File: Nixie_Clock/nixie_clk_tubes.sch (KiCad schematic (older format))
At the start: 20 parts, among them Y1 IN-14, Y2 IN-14, Y3 IN-14, Y4 IN-14, Y5 IN-14, Y6 IN-14, Y7 nixie_colon, Y8 nixie_colon

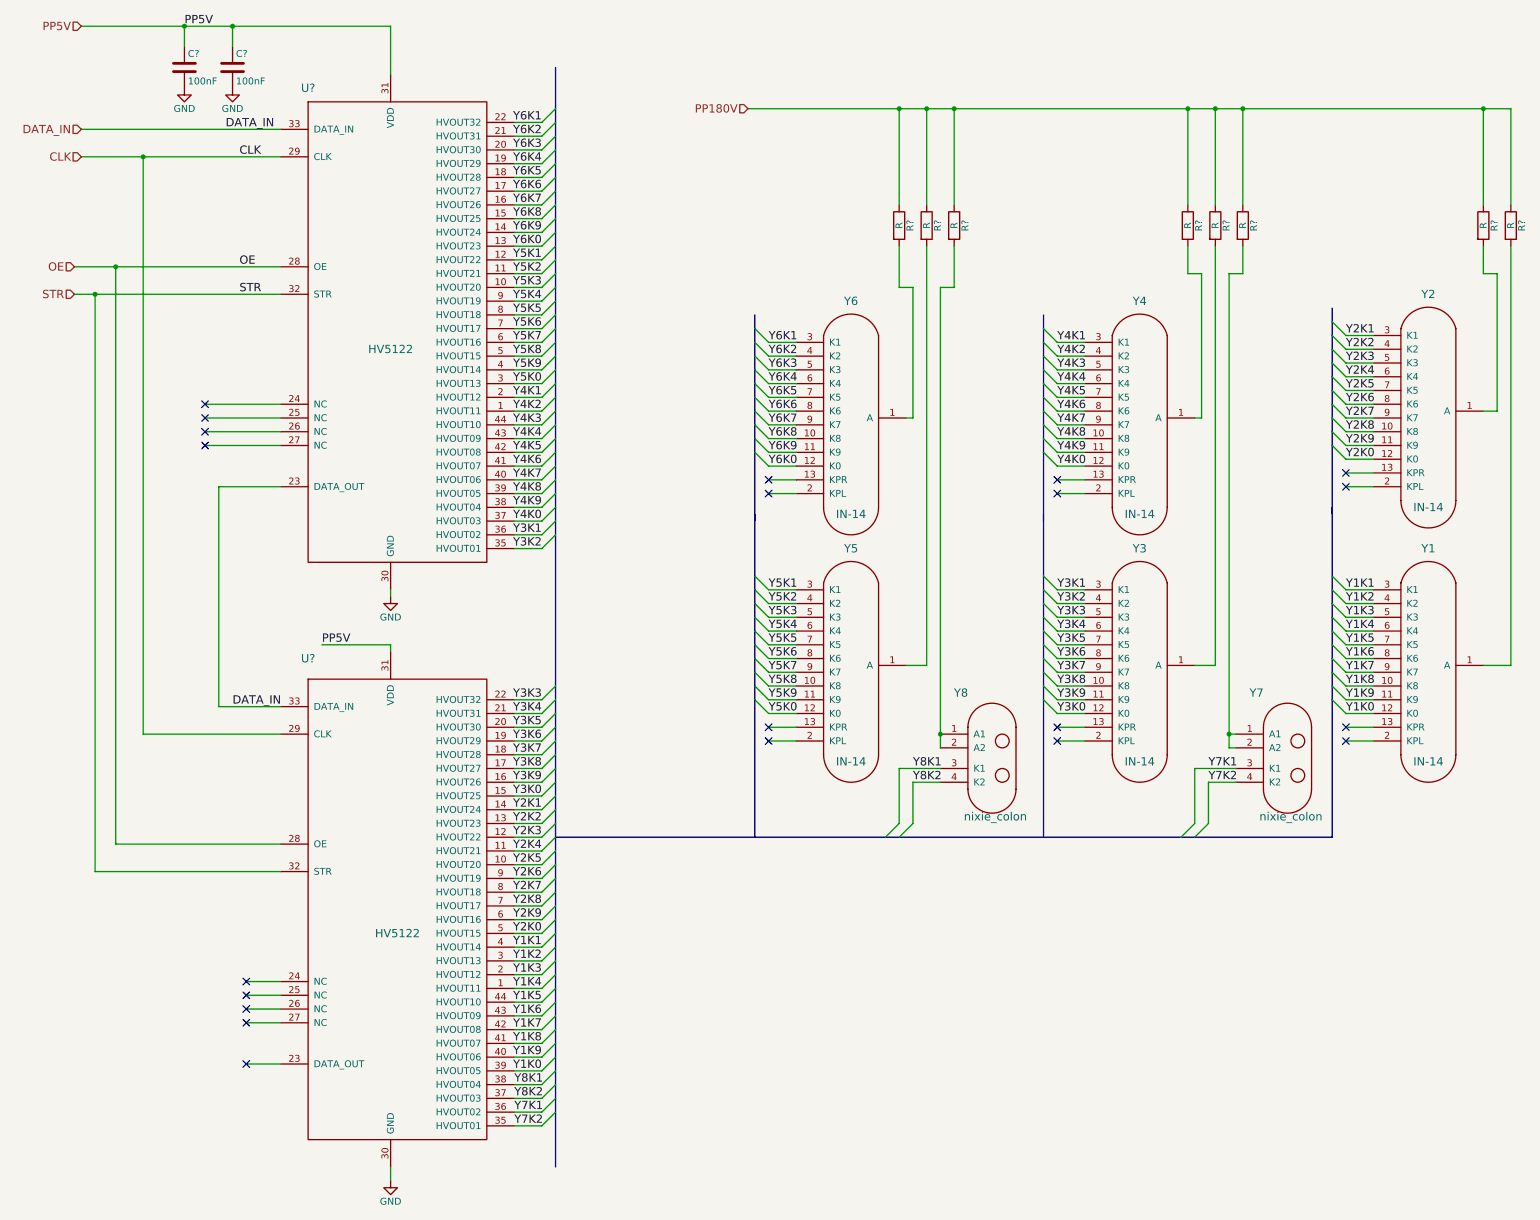
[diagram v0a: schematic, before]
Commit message: Sync remote
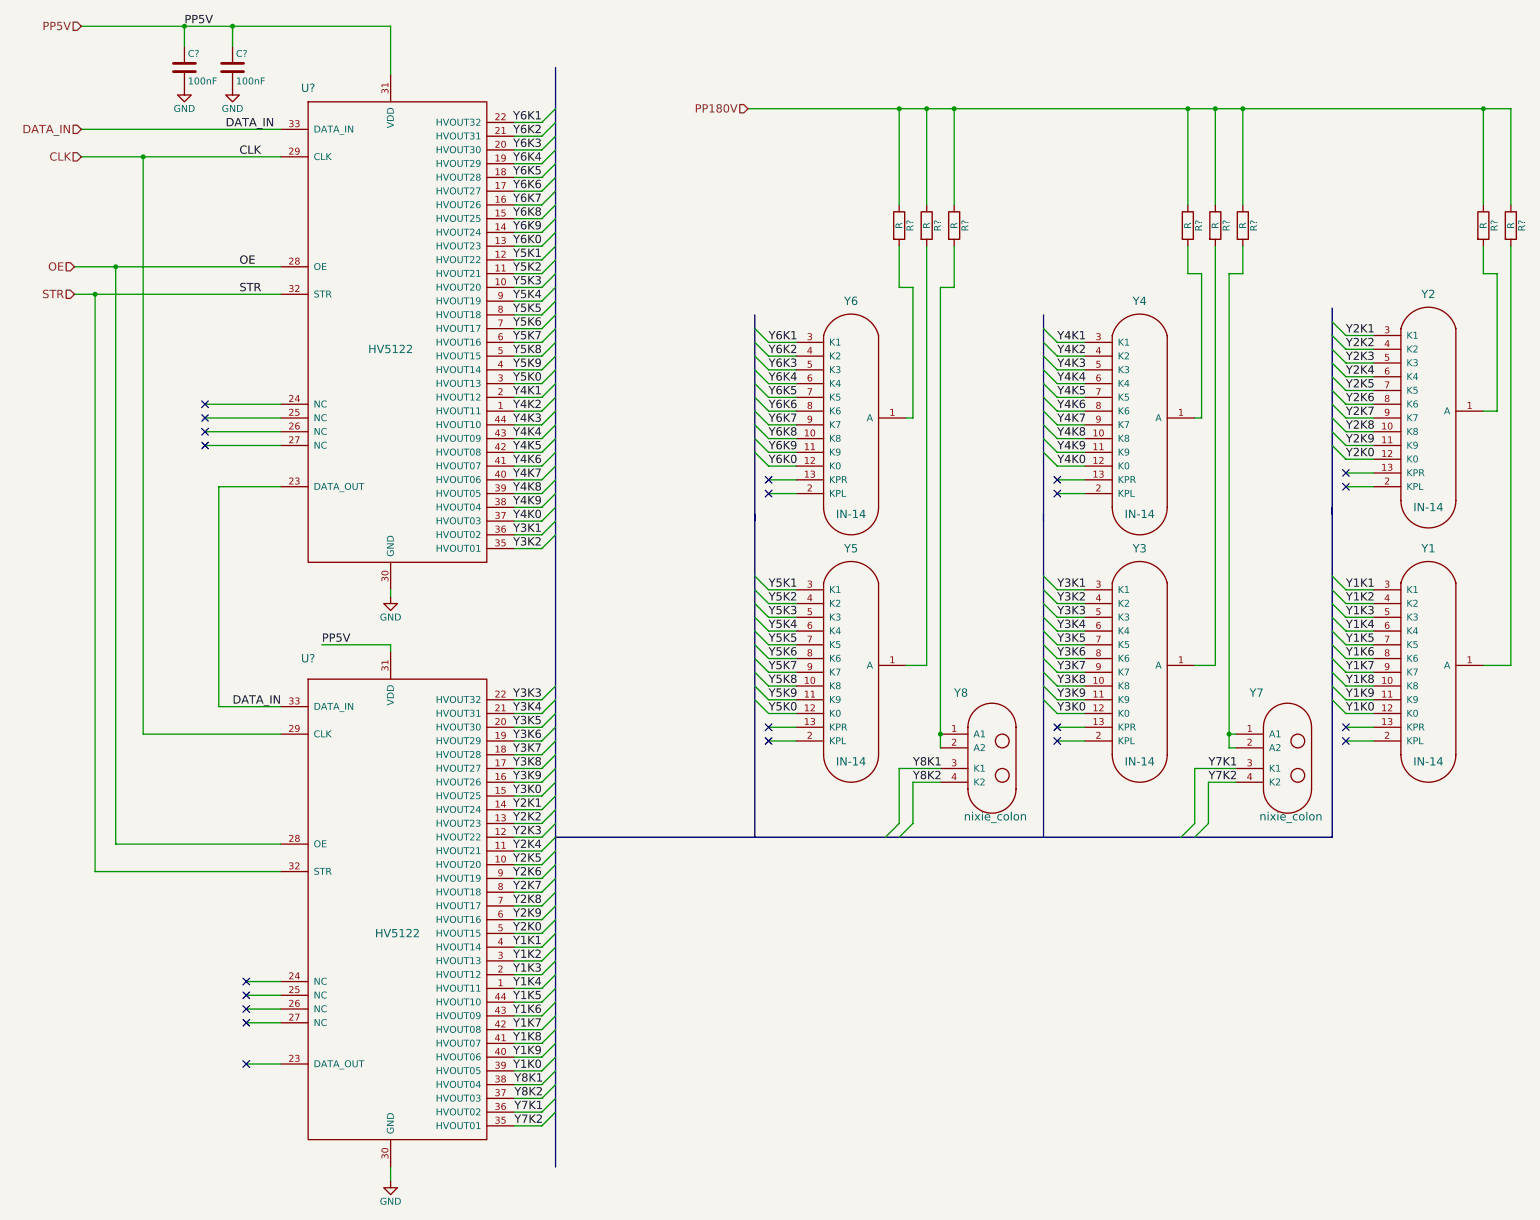
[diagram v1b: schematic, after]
